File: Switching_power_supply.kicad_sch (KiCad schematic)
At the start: 20 parts, among them J10 Conn_01x02, J12 Conn_01x02, J8 Conn_01x03_Pin, J9 Conn_01x02, U4 AMS1117, U5 LM2596HVS-ADJRG

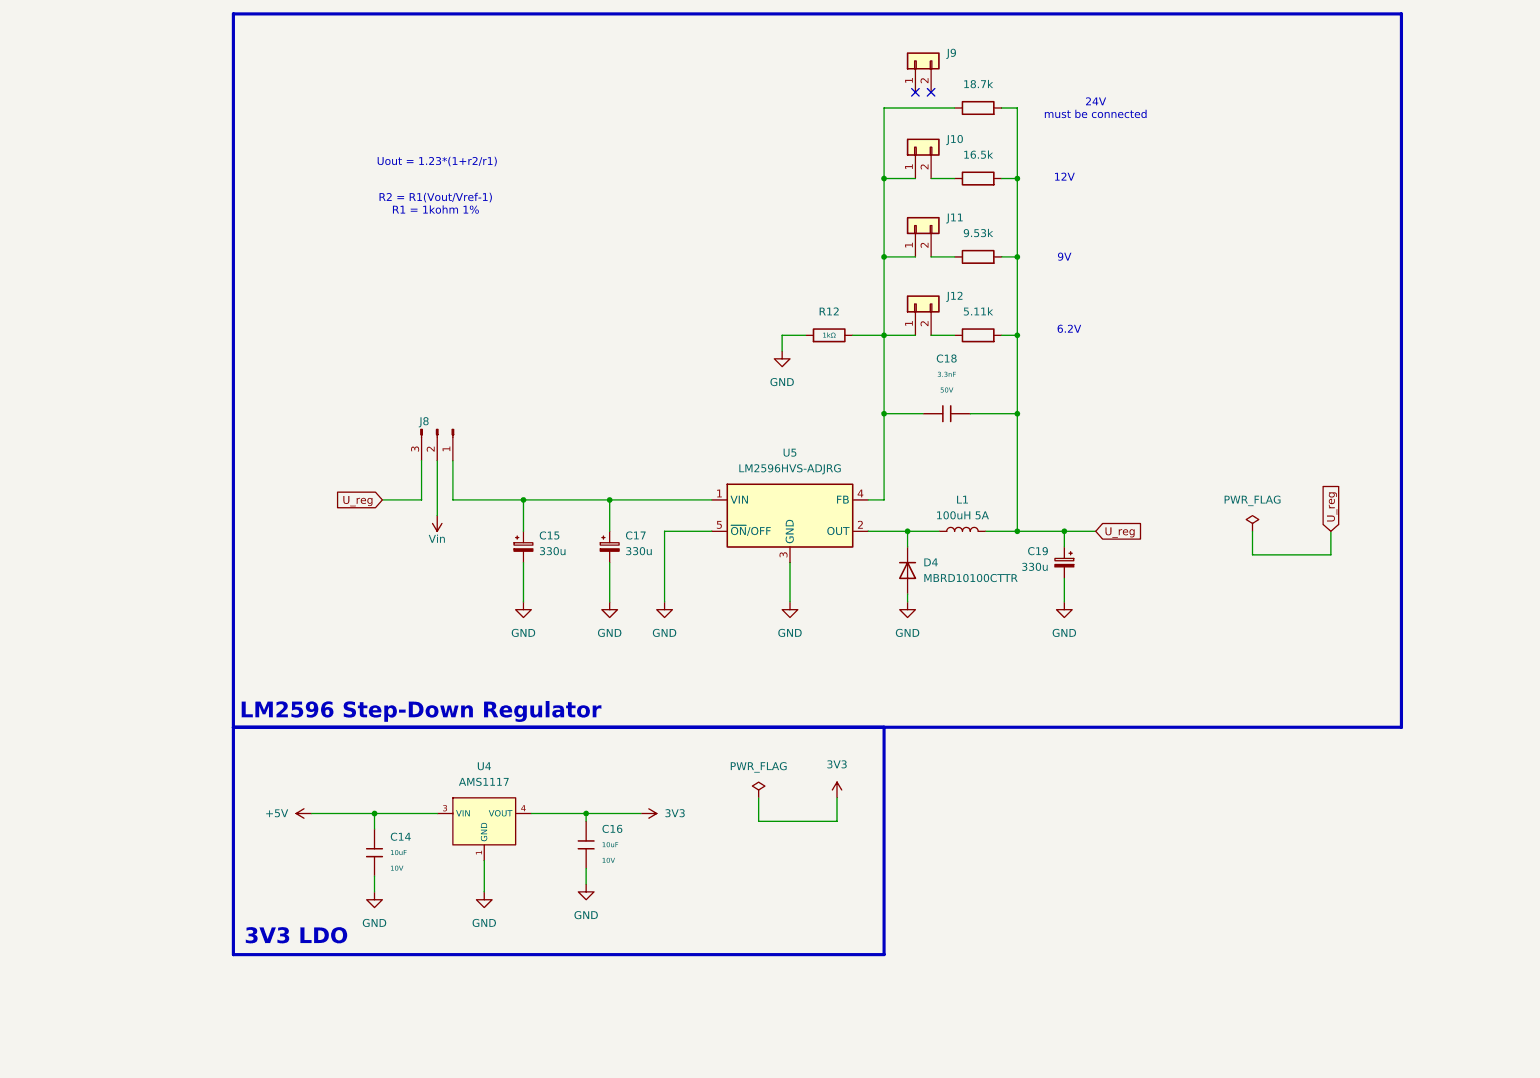
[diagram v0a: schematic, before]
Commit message: revision
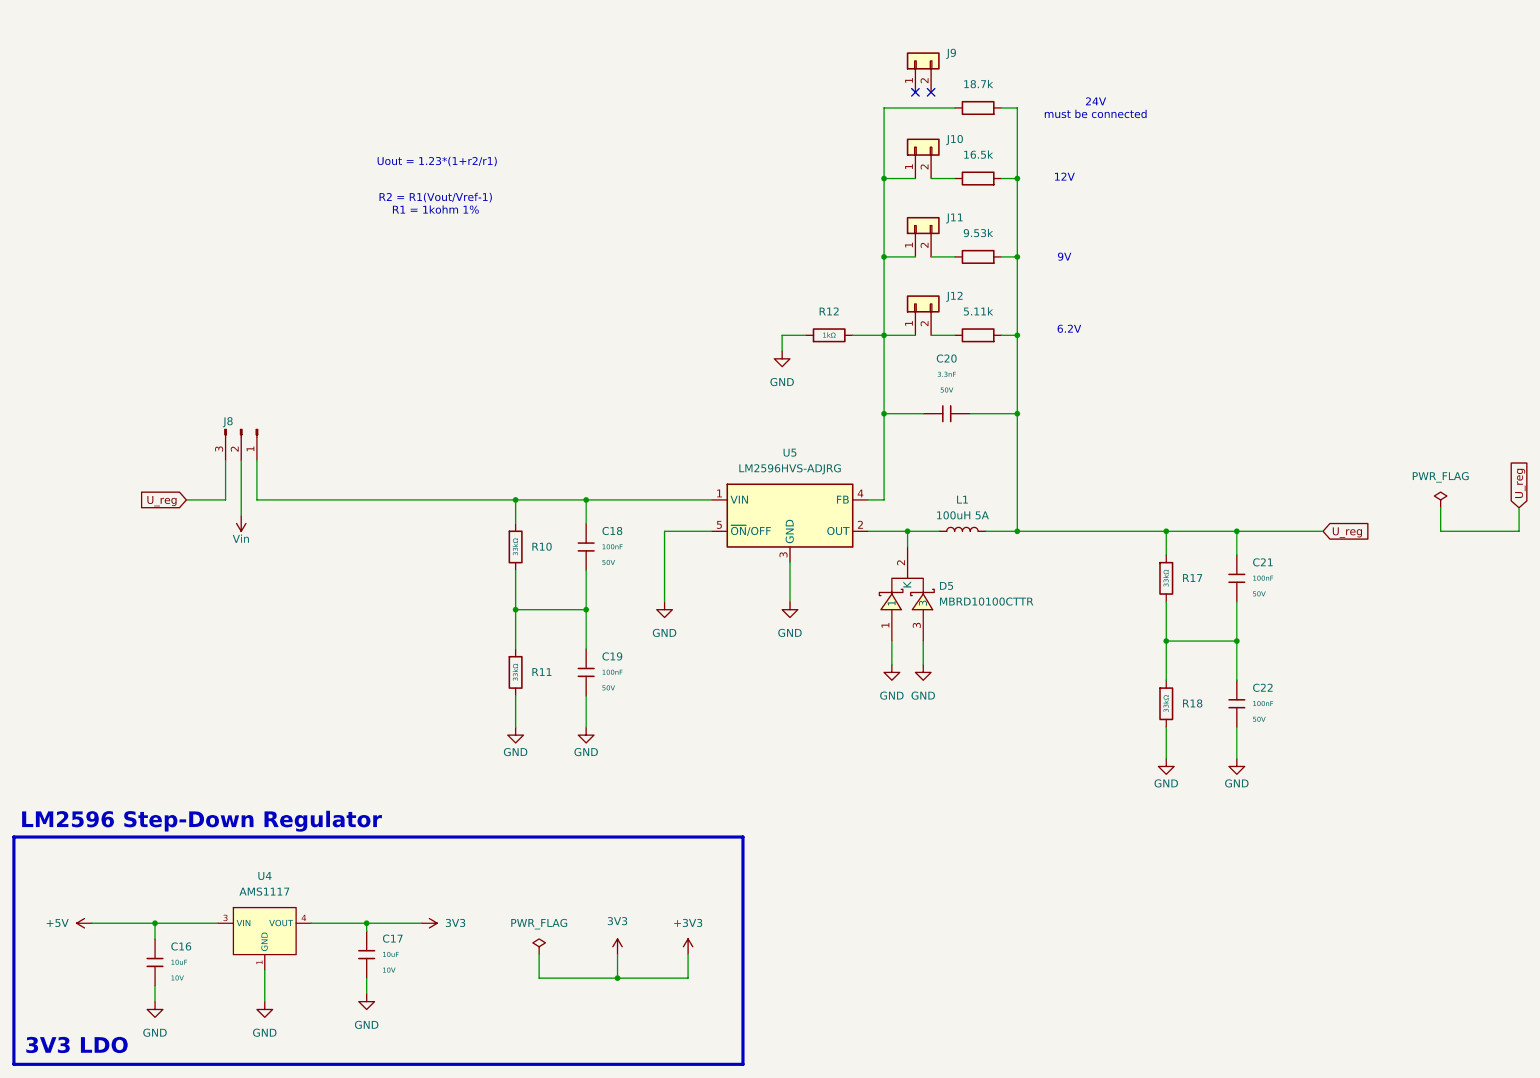
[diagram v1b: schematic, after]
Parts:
- removed C15, C17: 330u, Capacitor_THT:CP_Radial_D12.5mm_P5.00mm, symbol Device:C_Polarized_Small
- removed C19: 330u, Capacitor_SMD:CP_Elec_18x17.5, symbol Device:C_Polarized_Small
- removed D4: MBRD10100CTTR, Package_TO_SOT_SMD:TO-252-2, symbol Device:D
- added C18, C19, C21, C22: 100nF, PCM_JLCPCB:C_0603, symbol PCM_JLCPCB-Capacitors:0603,100nF
- added D5: MBRD10100CTTR, SMC_MBRD10100CTTR:TO-252-3_L6.5-W5.8-P4.58-TL, symbol SMC_MBRD10100CTTR:MBRD10100CTTR
- added R10, R11, R17, R18: 33kΩ, PCM_JLCPCB:R_0402, symbol PCM_JLCPCB-Resistors:0402,33kΩ
- J10, J12, J9: footprint Connector_PinHeader_2.54mm:PinHeader_1x02_P2.54mm_Vertical_SMD_Pin1Right -> Connector_PinHeader_2.54mm:PinHeader_1x02_P2.54mm_Vertical
- J11: value ~ -> Conn_01x02; footprint Connector_PinHeader_2.54mm:PinHeader_1x02_P2.54mm_Vertical_SMD_Pin1Right -> Connector_PinHeader_2.54mm:PinHeader_1x02_P2.54mm_Vertical
- R13: LCSC RC0402FR-0710KL -> C11476
- R14: LCSC FRC0402F1652TS -> C25857
- renumbered C14 to C16, C16 to C17, C18 to C20
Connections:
- net GND: now also C19.2, C22.2, D5.1, D5.3, R11.2, R18.2
- net U_reg: now also C21.1, R17.1
- net at L1.1, U5.2 (OUT): now also D5.2 (K)
- net at J8.1 (Pin_1), U5.1 (VIN): now also C18.1, R10.1
- net 3V3 renamed +3V3
- new net: C18.2, C19.1, R10.2, R11.1
- new net: C21.2, C22.1, R17.2, R18.1
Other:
- moved on the sheet: C16, C17, J8, U4
